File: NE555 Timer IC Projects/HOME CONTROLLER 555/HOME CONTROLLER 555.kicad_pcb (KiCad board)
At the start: 2 copper layers, 52 parts, among them J1 FAN, J2 PIR CONTROLLER, J3 POWER SUPPLY, J4 LIGHT, J5 Conn_01x06, J6 Conn_01x06, K1 SANYOU_SRD_Form_A, K2 SANYOU_SRD_Form_A, K3 SANYOU_SRD_Form_A, Q1 AO3400A, Q2 AO3400A, Q3 AO3400A, SW1 SW_Push, SW2 SW_Push, U1 ESP32-WROOM-32, U2 LM555xM, U3 LM393, U4 LM358, U6 AMS1117-3.3, U7 LM35-LP

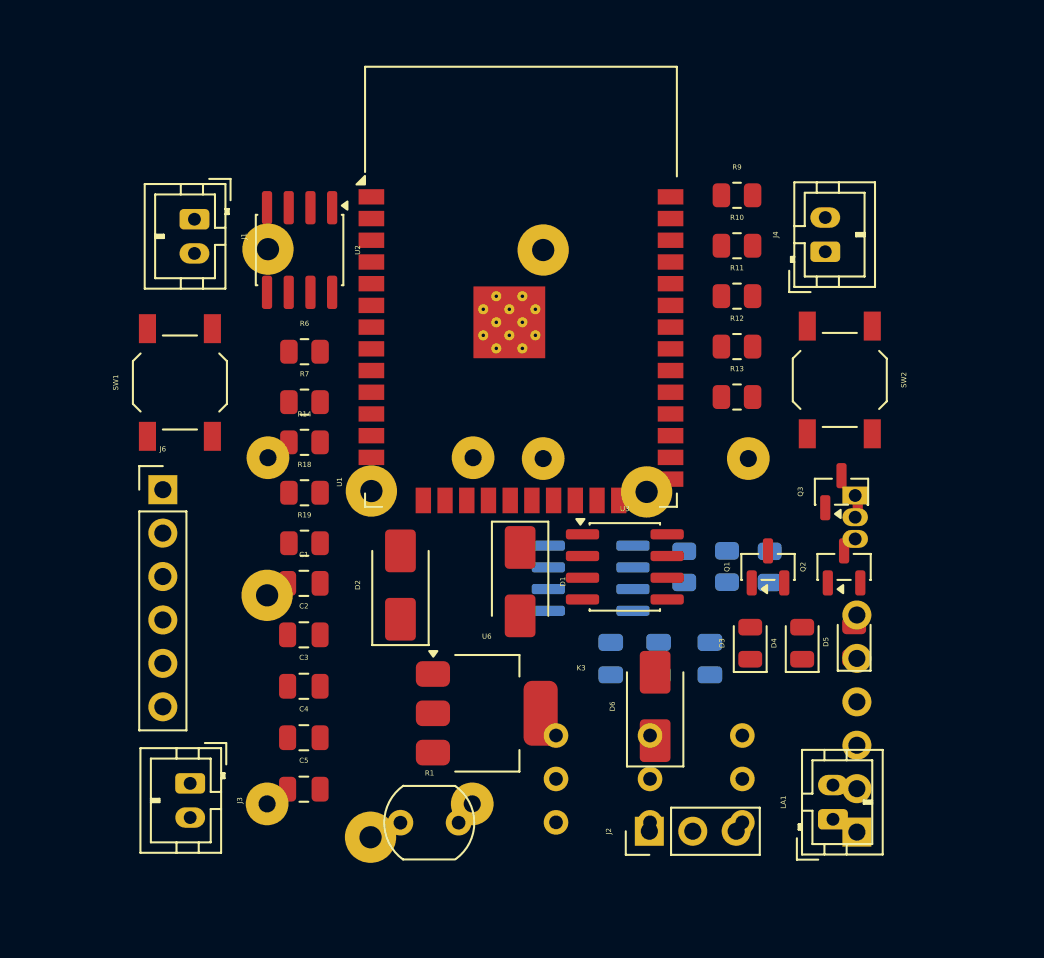
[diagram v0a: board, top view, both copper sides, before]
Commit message: Initial Commit
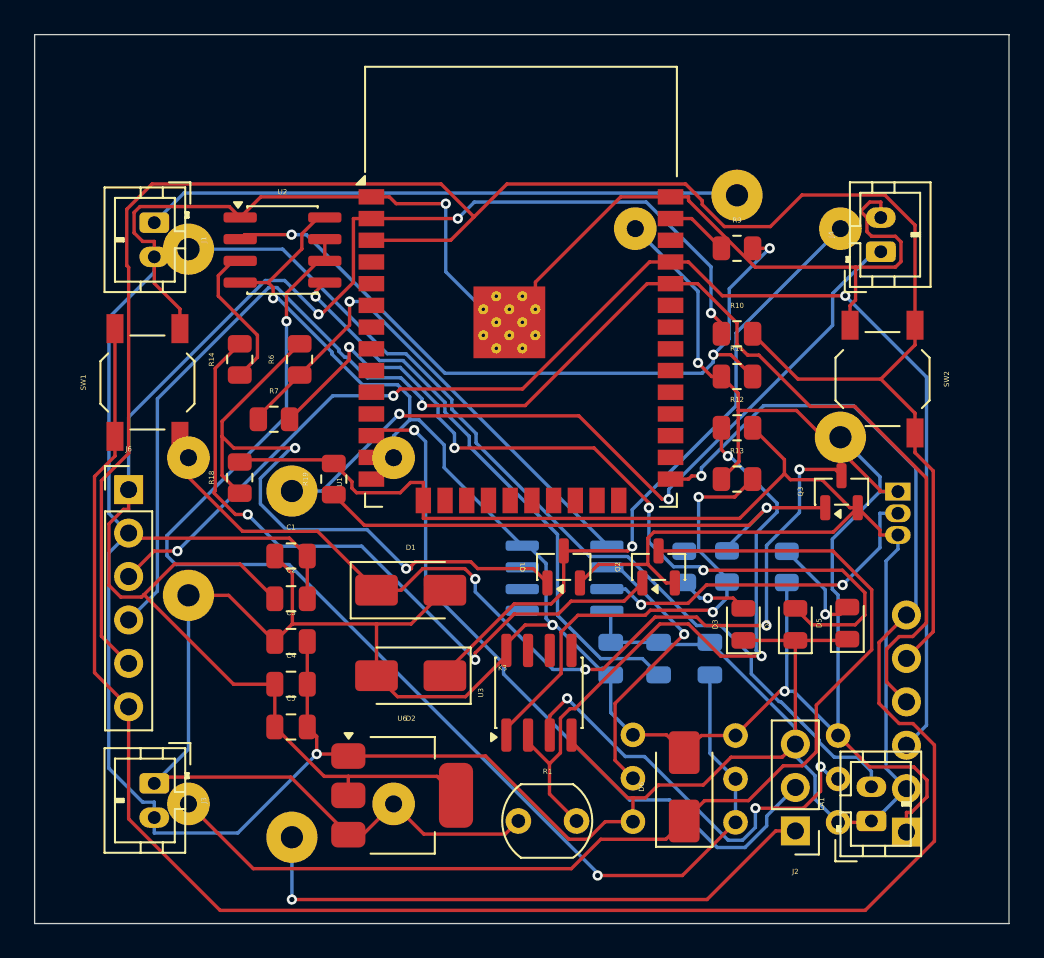
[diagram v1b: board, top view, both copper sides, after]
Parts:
- moved K2 18.1 mm to (201.6, 64.4), turned to -90 degrees
- moved Q1 12.0 mm to (191.4, 86.1)
- moved Q2 10.8 mm to (197.0, 86.1)
- moved U3 8.92 mm to (190.0, 93.5), turned to 90 degrees
- moved J2 8.54 mm to (205.0, 101.6), turned to 180 degrees
- moved R1 6.90 mm to (188.8, 101.0)
- moved U6 6.90 mm to (182.0, 99.5)
- moved D1 6.42 mm to (182.5, 87.5), turned to 0 degrees
- moved R14 6.15 mm to (172.5, 74.0), turned to 90 degrees
- moved RV1 5.60 mm to (207.5, 96.0)
- moved D2 5.33 mm to (182.5, 92.5), turned to 180 degrees
- moved R10 5.15 mm to (201.6, 72.5)
- moved RV2 5.00 mm to (201.5, 96.0)
- moved D6 5.00 mm to (198.5, 99.0)
- moved R13 4.80 mm to (201.6, 81.0)
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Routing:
- net GND: track 0.00 -> 322.8 mm, vias 0 -> 2
- net +5V: track 0.00 -> 202.7 mm, vias 0 -> 4
- net GPIO0: track 0.00 -> 123.5 mm, vias 0 -> 1
- net EN: track 0.00 -> 122.2 mm
- net 3V3: track 0.00 -> 96.7 mm, vias 0 -> 3
- net GPIO3: track 0.00 -> 87.9 mm, vias 0 -> 1
- net GPIO1: track 0.00 -> 79.1 mm, vias 0 -> 3
- net U2 PIN6&7: track 0.00 -> 74.2 mm, vias 0 -> 2
- net Net-(D6-K): track 0.00 -> 65.4 mm
- net Net-(D1-K): track 0.00 -> 55.1 mm, vias 0 -> 4
- net Net-(LA1-+): track 0.00 -> 54.8 mm
- net Net-(D4-A): track 0.00 -> 50.0 mm, vias 0 -> 4
- net Net-(J4-Pin_1): track 0.00 -> 45.8 mm, vias 0 -> 2
- net Net-(U2-TR): track 0.00 -> 43.3 mm, vias 0 -> 3
- net GPIO27: track 0.00 -> 42.1 mm, vias 0 -> 1
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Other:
- board outline added: 57 x 52 mm
